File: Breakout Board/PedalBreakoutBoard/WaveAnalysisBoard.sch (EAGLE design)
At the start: 53 parts, among them IC1 LD1117V, IC2 MCP6004P, U1 OPA1652AID

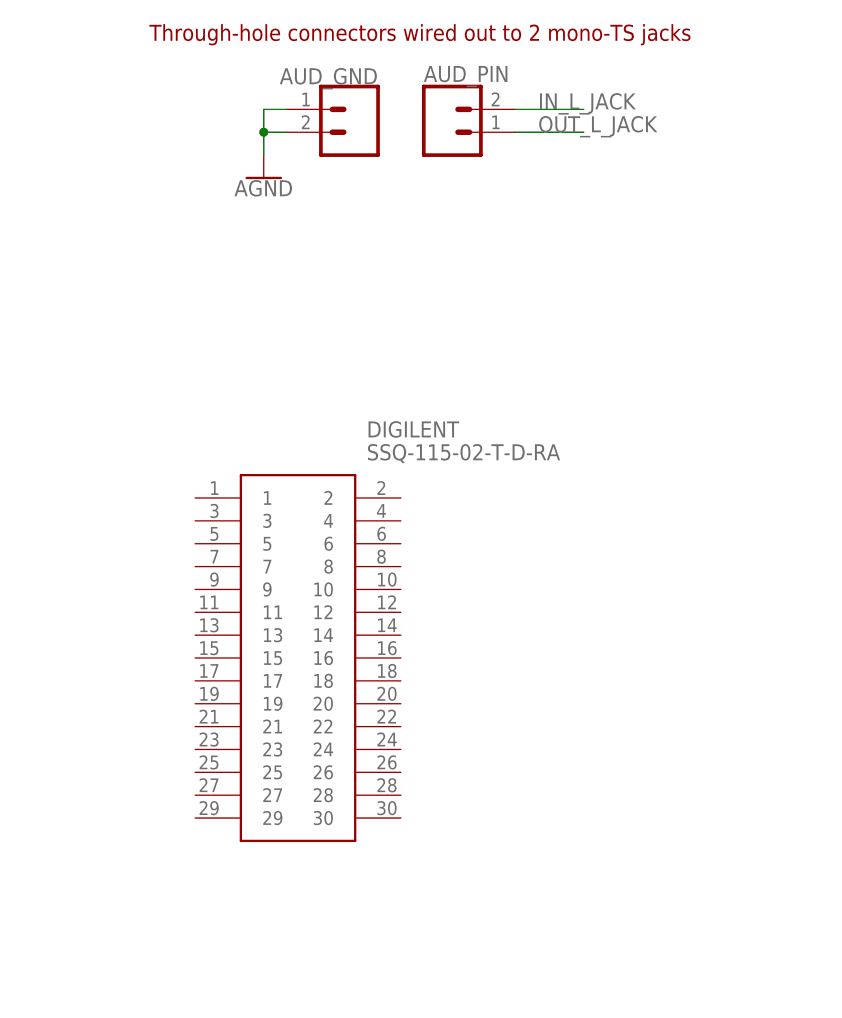
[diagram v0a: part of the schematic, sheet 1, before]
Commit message: DP-97 - Working on adding header
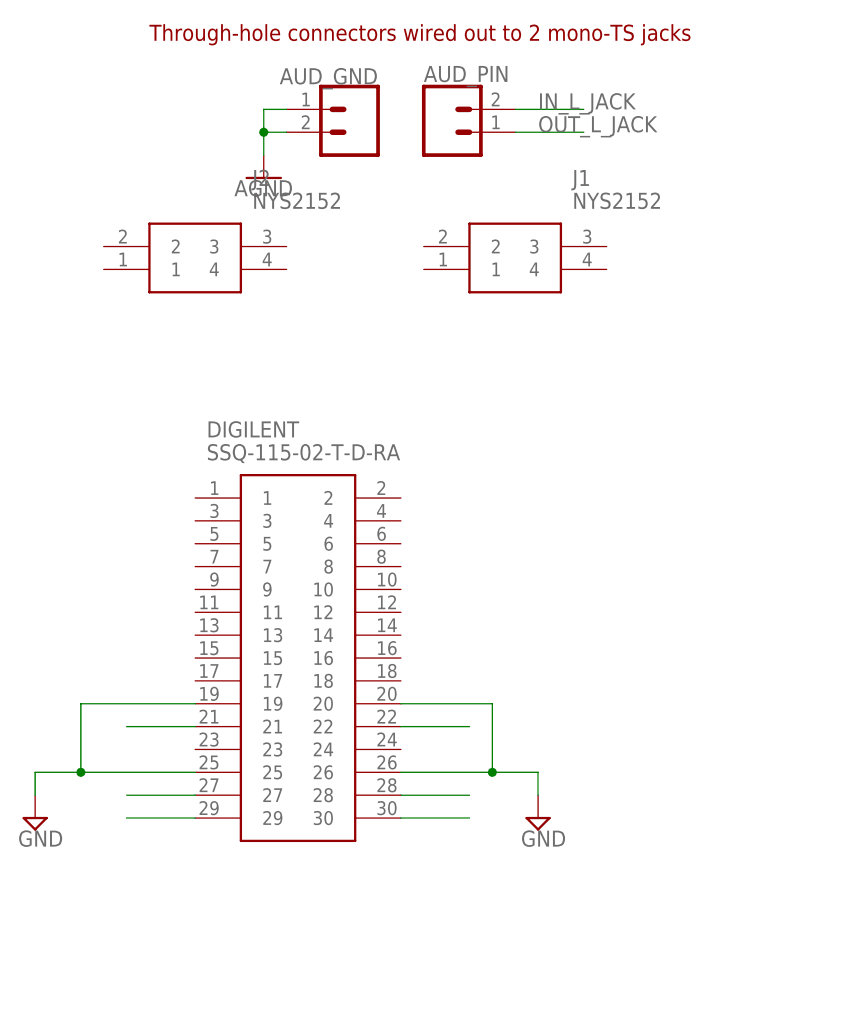
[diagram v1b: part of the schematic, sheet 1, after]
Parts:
- added J1, J2: NYS2152, SamacSys_Parts:NYS2152
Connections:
- new net N$11: DIGILENT.21
- new net N$16: DIGILENT.22
- new net N$17: DIGILENT.28
- new net N$19: DIGILENT.30
- new net N$20: DIGILENT.27
- new net N$21: DIGILENT.29
- net GND: now also DIGILENT.19, DIGILENT.20, DIGILENT.25, DIGILENT.26
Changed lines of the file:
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@@
 <schematic_group name="AUDIO_INPUT"/>
 <schematic_group name="AUDIO_PWR"/>
-<schematic_group name="AUDIO_JACKS"/>
 </groups>
 <parts>
@@
 <part name="SUPPLY6" library="supply2" library_urn="urn:adsk.eagle:library:372" deviceset="GND" device=""/>
 <part name="DIGILENT" library="SamacSys_Parts" deviceset="SSQ-115-02-T-D-RA" device=""/>
+<part name="SUPPLY7" library="supply2" library_urn="urn:adsk.eagle:library:372" deviceset="GND" device=""/>
+<part name="SUPPLY8" library="supply2" library_urn="urn:adsk.eagle:library:372" deviceset="GND" device=""/>
+<part name="J1" library="SamacSys_Parts" deviceset="NYS2152" device=""/>
+<part name="J2" library="SamacSys_Parts" deviceset="NYS2152" device=""/>
 </parts>
 <sheets>
@@
 <description>Audio &amp; Power</description>
 <plain>
-<text x="-20.32" y="157.48" size="1.778" layer="94" grouprefs="AUDIO_JACKS">Through-hole connectors wired out to 2 mono-TS jacks</text>
+<text x="-20.32" y="157.48" size="1.778" layer="94">Through-hole connectors wired out to 2 mono-TS jacks</text>
 <text x="7.62" y="25.4" size="1.778" layer="94" grouprefs="POWER">This section provides connection to a 9V
 barrel jack, feeding the V_IN pin on the Seed
@@
 <attribute name="VALUE" x="246.38" y="110.744" size="1.778" layer="96" font="vector" rot="R180" align="top-center"/>
 </instance>
-<instance part="AUD_PIN" gate="G$1" x="12.7" y="147.32" smashed="yes" grouprefs="AUDIO_JACKS">
+<instance part="AUD_PIN" gate="G$1" x="12.7" y="147.32" smashed="yes">
 <attribute name="VALUE" x="10.16" y="142.494" size="1.778" layer="96" font="vector"/>
 <attribute name="NAME" x="10.16" y="152.908" size="1.778" layer="95" font="vector"/>
 </instance>
-<instance part="AUD_GND" gate="G$1" x="2.54" y="149.86" smashed="yes" rot="R180" grouprefs="AUDIO_JACKS">
+<instance part="AUD_GND" gate="G$1" x="2.54" y="149.86" smashed="yes" rot="R180">
 <attribute name="VALUE" x="5.08" y="154.686" size="1.778" layer="96" font="vector" rot="R180"/>
 <attribute name="NAME" x="5.08" y="154.432" size="1.778" layer="95" font="vector" rot="R180"/>
@@
 <attribute name="VALUE" x="71.12" y="60.706" size="1.778" layer="96" align="top-center"/>
 </instance>
-<instance part="U$2" gate="G$1" x="-7.62" y="142.24" smashed="yes" grouprefs="AUDIO_JACKS">
+<instance part="U$2" gate="G$1" x="-7.62" y="142.24" smashed="yes">
 <attribute name="VALUE" x="-7.62" y="141.986" size="1.778" layer="96" align="top-center"/>
 </instance>
@@
 </instance>
 <instance part="DIGILENT" gate="G$1" x="-15.24" y="106.68" smashed="yes">
-<attribute name="NAME" x="3.81" y="114.3" size="1.778" layer="95" align="center-left"/>
-<attribute name="VALUE" x="3.81" y="111.76" size="1.778" layer="96" align="center-left"/>
+<attribute name="NAME" x="-13.97" y="114.3" size="1.778" layer="95" align="center-left"/>
+<attribute name="VALUE" x="-13.97" y="111.76" size="1.778" layer="96" align="center-left"/>
+</instance>
+<instance part="SUPPLY7" gate="GND" x="22.86" y="71.12" smashed="yes">
+<attribute name="VALUE" x="20.955" y="67.945" size="1.778" layer="96"/>
+</instance>
+<instance part="SUPPLY8" gate="GND" x="-33.02" y="71.12" smashed="yes">
+<attribute name="VALUE" x="-34.925" y="67.945" size="1.778" layer="96"/>
+</instance>
+<instance part="J1" gate="G$1" x="10.16" y="134.62" smashed="yes">
+<attribute name="NAME" x="26.67" y="142.24" size="1.778" layer="95" align="center-left"/>
+<attribute name="VALUE" x="26.67" y="139.7" size="1.778" layer="96" align="center-left"/>
+</instance>
+<instance part="J2" gate="G$1" x="-25.4" y="134.62" smashed="yes">
+<attribute name="NAME" x="-8.89" y="142.24" size="1.778" layer="95" align="center-left"/>
+<attribute name="VALUE" x="-8.89" y="139.7" size="1.778" layer="96" align="center-left"/>
 </instance>
 </instances>
@@
 <pinref part="C6" gate="G$1" pin="2"/>
 </segment>
+<segment>
+<pinref part="DIGILENT" gate="G$1" pin="20"/>
+<wire x1="7.62" y1="83.82" x2="17.78" y2="83.82" width="0.1524" layer="91"/>
+<pinref part="DIGILENT" gate="G$1" pin="26"/>
+<wire x1="7.62" y1="76.2" x2="17.78" y2="76.2" width="0.1524" layer="91"/>
+<wire x1="17.78" y1="83.82" x2="17.78" y2="76.2" width="0.1524" layer="91"/>
+<junction x="17.78" y="76.2"/>
+<wire x1="17.78" y1="76.2" x2="22.86" y2="76.2" width="0.1524" layer="91"/>
+<wire x1="22.86" y1="76.2" x2="22.86" y2="73.66" width="0.1524" layer="91"/>
+<pinref part="SUPPLY7" gate="GND" pin="GND"/>
+</segment>
+<segment>
+<pinref part="DIGILENT" gate="G$1" pin="19"/>
+<wire x1="-15.24" y1="83.82" x2="-27.94" y2="83.82" width="0.1524" layer="91"/>
+<wire x1="-27.94" y1="83.82" x2="-27.94" y2="76.2" width="0.1524" layer="91"/>
+<pinref part="DIGILENT" gate="G$1" pin="25"/>
+<wire x1="-27.94" y1="76.2" x2="-15.24" y2="76.2" width="0.1524" layer="91"/>
+<wire x1="-27.94" y1="76.2" x2="-33.02" y2="76.2" width="0.1524" layer="91"/>
+<junction x="-27.94" y="76.2"/>
+<wire x1="-33.02" y1="76.2" x2="-33.02" y2="73.66" width="0.1524" layer="91"/>
+<pinref part="SUPPLY8" gate="GND" pin="GND"/>
+</segment>
 </net>
 <net name="SPST1" class="0">
@@
 <net name="IN_L_JACK" class="0">
 <segment>
-<wire x1="20.32" y1="149.86" x2="27.94" y2="149.86" width="0.1524" layer="91" grouprefs="AUDIO_JACKS"/>
-<label x="22.86" y="149.86" size="1.778" layer="95" grouprefs="AUDIO_JACKS"/>
+<wire x1="20.32" y1="149.86" x2="27.94" y2="149.86" width="0.1524" layer="91"/>
+<label x="22.86" y="149.86" size="1.778" layer="95"/>
 <pinref part="AUD_PIN" gate="G$1" pin="2"/>
 </segment>
@@
 <net name="OUT_L_JACK" class="0">
 <segment>
-<wire x1="20.32" y1="147.32" x2="27.94" y2="147.32" width="0.1524" layer="91" grouprefs="AUDIO_JACKS"/>
-<label x="22.86" y="147.32" size="1.778" layer="95" grouprefs="AUDIO_JACKS"/>
+<wire x1="20.32" y1="147.32" x2="27.94" y2="147.32" width="0.1524" layer="91"/>
+<label x="22.86" y="147.32" size="1.778" layer="95"/>
 <pinref part="AUD_PIN" gate="G$1" pin="1"/>
 </segment>
@@
 <segment>
 <pinref part="AUD_GND" gate="G$1" pin="1"/>
-<wire x1="-5.08" y1="149.86" x2="-7.62" y2="149.86" width="0.1524" layer="91" grouprefs="AUDIO_JACKS"/>
-<wire x1="-7.62" y1="149.86" x2="-7.62" y2="147.32" width="0.1524" layer="91" grouprefs="AUDIO_JACKS"/>
+<wire x1="-5.08" y1="149.86" x2="-7.62" y2="149.86" width="0.1524" layer="91"/>
+<wire x1="-7.62" y1="149.86" x2="-7.62" y2="147.32" width="0.1524" layer="91"/>
 <pinref part="AUD_GND" gate="G$1" pin="2"/>
-<wire x1="-7.62" y1="147.32" x2="-7.62" y2="144.78" width="0.1524" layer="91" grouprefs="AUDIO_JACKS"/>
-<wire x1="-5.08" y1="147.32" x2="-7.62" y2="147.32" width="0.1524" layer="91" grouprefs="AUDIO_JACKS"/>
-<junction x="-7.62" y="147.32" grouprefs="AUDIO_JACKS"/>
+<wire x1="-7.62" y1="147.32" x2="-7.62" y2="144.78" width="0.1524" layer="91"/>
+<wire x1="-5.08" y1="147.32" x2="-7.62" y2="147.32" width="0.1524" layer="91"/>
+<junction x="-7.62" y="147.32"/>
 <pinref part="U$2" gate="G$1" pin="AGND"/>
 </segment>
@@
 </segment>
 </net>
+<net name="N$11" class="0">
+<segment>
+<pinref part="DIGILENT" gate="G$1" pin="21"/>
+<wire x1="-15.24" y1="81.28" x2="-22.86" y2="81.28" width="0.1524" layer="91"/>
+</segment>
+</net>
+<net name="N$16" class="0">
+<segment>
+<pinref part="DIGILENT" gate="G$1" pin="22"/>
+<wire x1="7.62" y1="81.28" x2="15.24" y2="81.28" width="0.1524" layer="91"/>
+</segment>
+</net>
+<net name="N$17" class="0">
+<segment>
+<pinref part="DIGILENT" gate="G$1" pin="28"/>
+<wire x1="7.62" y1="73.66" x2="15.24" y2="73.66" width="0.1524" layer="91"/>
+</segment>
+</net>
+<net name="N$19" class="0">
+<segment>
+<pinref part="DIGILENT" gate="G$1" pin="30"/>
+<wire x1="7.62" y1="71.12" x2="15.24" y2="71.12" width="0.1524" layer="91"/>
+</segment>
+</net>
+<net name="N$20" class="0">
+<segment>
+<pinref part="DIGILENT" gate="G$1" pin="27"/>
+<wire x1="-15.24" y1="73.66" x2="-22.86" y2="73.66" width="0.1524" layer="91"/>
+</segment>
+</net>
+<net name="N$21" class="0">
+<segment>
+<pinref part="DIGILENT" gate="G$1" pin="29"/>
+<wire x1="-15.24" y1="71.12" x2="-22.86" y2="71.12" width="0.1524" layer="91"/>
+</segment>
+</net>
